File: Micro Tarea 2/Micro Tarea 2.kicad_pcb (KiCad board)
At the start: 4 copper layers, 70.8 x 86.7 mm, 62 parts, among them J1 Screw_Terminal_01x02, P1 USB_C_Plug_USB2.0, U7 TPS62130, U8 ESP32-S3R8, U9 W25Q128JVSIQ, Y1 40MHz

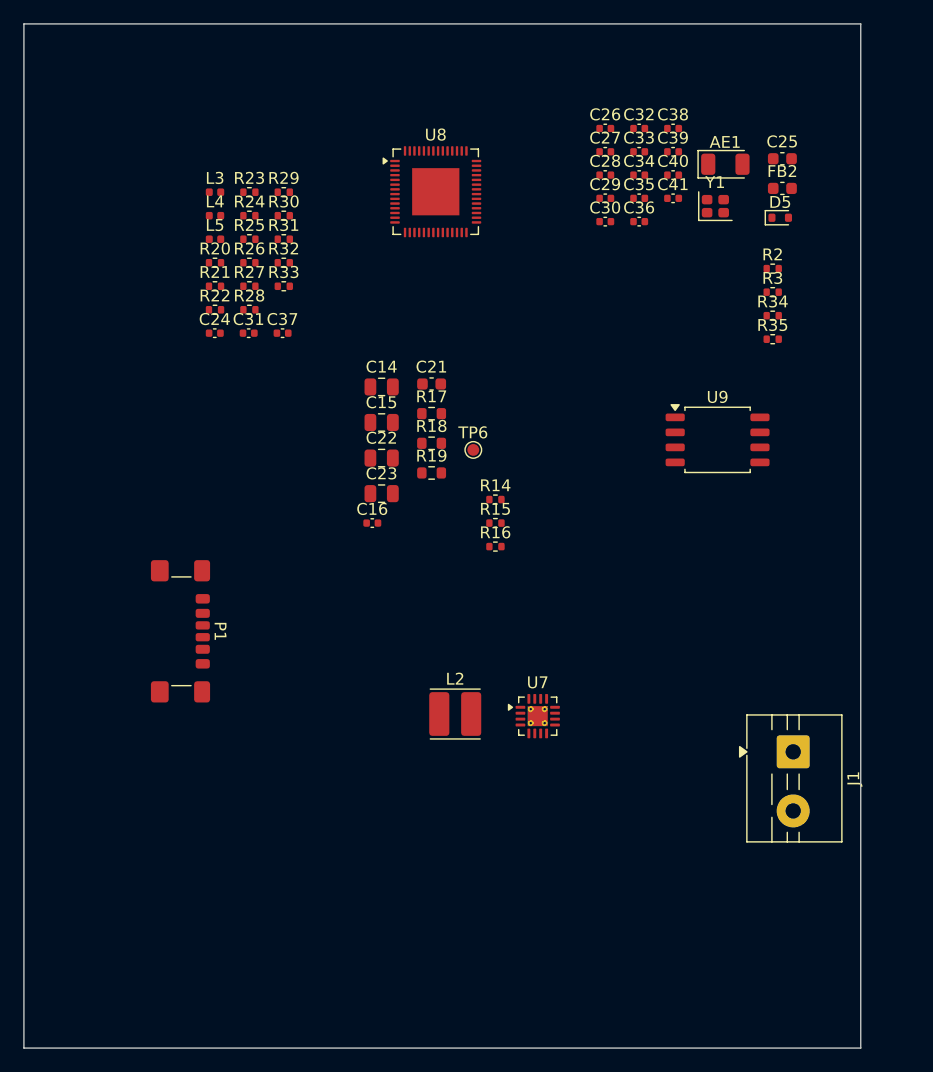
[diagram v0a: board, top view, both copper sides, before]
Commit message: actualizando placa
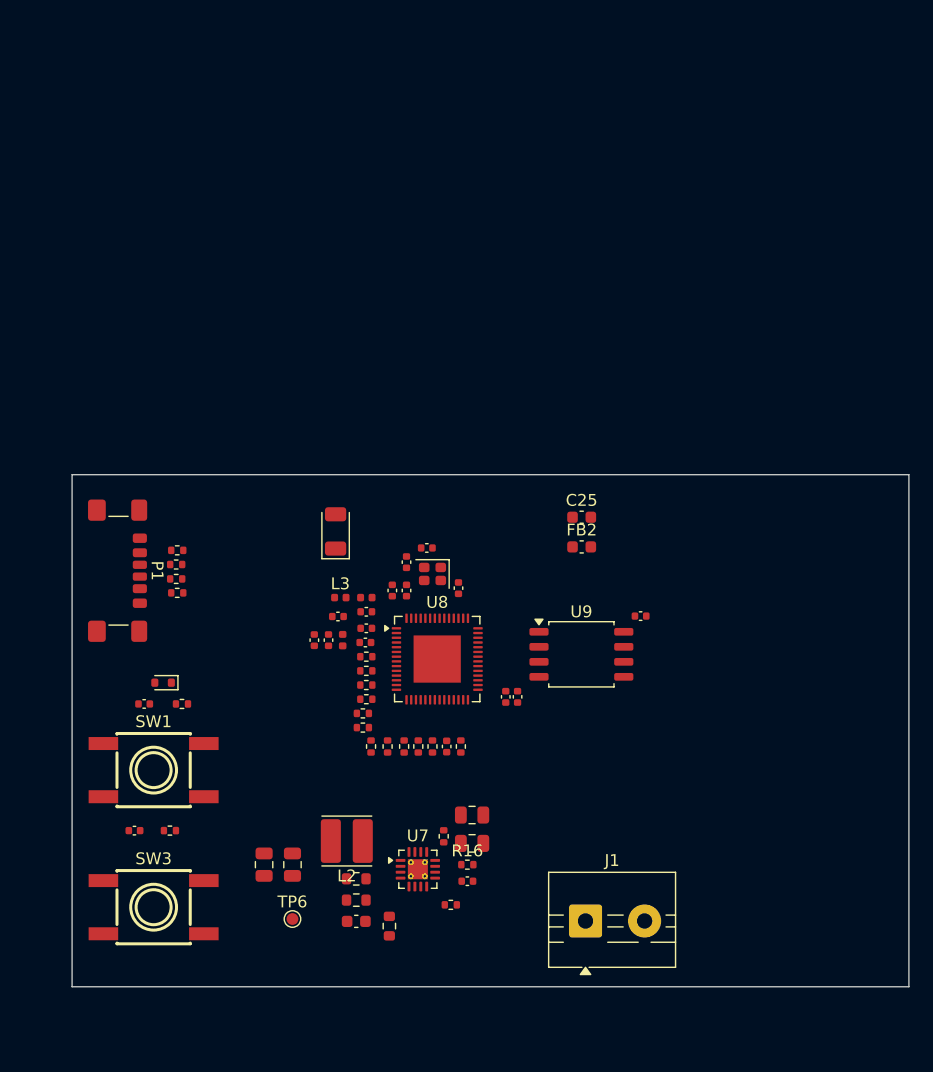
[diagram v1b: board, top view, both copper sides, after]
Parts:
- added SW1: K2-1157SP-I4SW-04, JLCImport:K2-1157SP-I4SW-04, F.Cu at (117.3, 101.5)
- added SW3: K2-1157SP-I4SW-04, JLCImport:K2-1157SP-I4SW-04, F.Cu at (117.3, 113.1)
- moved C29 66.7 mm to (115.7, 106.7), turned to 180 degrees
- moved D5 65.4 mm to (118.1, 94.1), turned to 180 degrees
- moved R2 57.4 mm to (119.3, 86.5)
- moved R3 54.9 mm to (119.3, 82.9)
- moved R34 54.7 mm to (119.2, 84.1)
- moved R35 54.4 mm to (119.2, 85.4)
- moved C39 50.6 mm to (132.1, 90.5), turned to -90 degrees
- moved C38 50.1 mm to (132.9, 88.5), turned to 180 degrees
- moved C40 49.7 mm to (130.9, 90.5), turned to -90 degrees
- moved C30 46.4 mm to (142.1, 99.5), turned to -90 degrees
- moved R21 46.2 mm to (118.7, 106.7), turned to 180 degrees
- moved C21 45.9 mm to (134.4, 114.3)
- moved C34 45.6 mm to (147.1, 95.3), turned to -90 degrees
- moved AE1 45.3 mm to (132.7, 81.3), turned to 90 degrees
- moved R23 45.1 mm to (135.0, 96.7), turned to 180 degrees
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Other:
- board size 70.8 x 86.7 mm -> 70.8 x 43.3 mm
